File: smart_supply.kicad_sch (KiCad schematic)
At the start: 0 parts

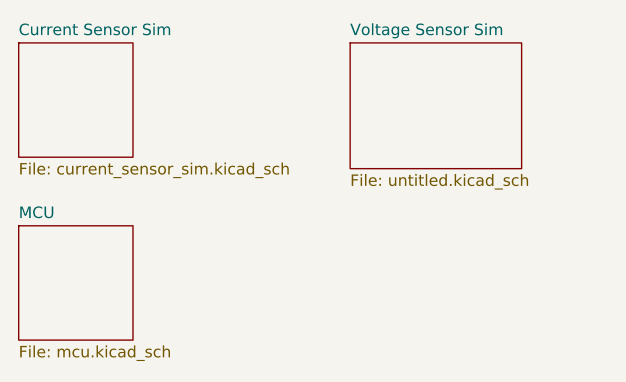
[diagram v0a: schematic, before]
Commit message: opamp chain fix
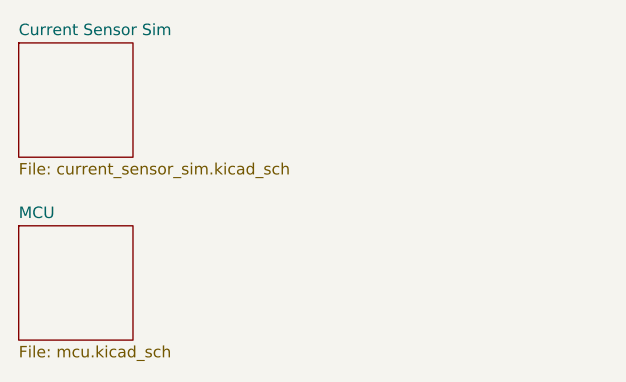
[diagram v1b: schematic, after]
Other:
- removed sheet Voltage Sensor Sim
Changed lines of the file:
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@@
-	)
-	(sheet
-		(at 59.69 21.59)
-		(size 19.05 13.97)
-		(exclude_from_sim no)
-		(in_bom yes)
-		(on_board yes)
-		(dnp no)
-		(fields_autoplaced yes)
-		(stroke
-			(width 0.1524)
-			(type solid)
-		)
-		(fill
-			(color 0 0 0 0)
-		)
-		(property "Sheetname" "Voltage Sensor Sim"
-			(at 59.69 20.8784 0)
-			(show_name no)
-			(do_not_autoplace no)
-			(effects
-				(font
-					(size 1.27 1.27)
-				)
-				(justify left bottom)
-			)
-		)
-		(property "Sheetfile" "untitled.kicad_sch"
-			(at 59.69 36.1446 0)
-			(show_name no)
-			(do_not_autoplace no)
-			(effects
-				(font
-					(size 1.27 1.27)
-				)
-				(justify left top)
-			)
-		)
-		(instances
-			(project "smart_supply"
-				(path "/487ef637-7a03-4925-80c1-798e0c6f0bbd"
-					(page "4")
-				)
-			)
-		)
 	)
 	(sheet

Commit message: built opamp network
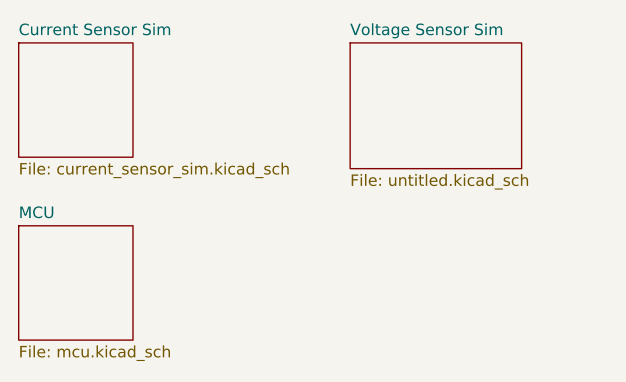
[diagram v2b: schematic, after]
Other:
- added sheet Voltage Sensor Sim (untitled.kicad_sch)
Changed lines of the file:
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@@
+	)
+	(sheet
+		(at 59.69 21.59)
+		(size 19.05 13.97)
+		(exclude_from_sim no)
+		(in_bom yes)
+		(on_board yes)
+		(dnp no)
+		(fields_autoplaced yes)
+		(stroke
+			(width 0.1524)
+			(type solid)
+		)
+		(fill
+			(color 0 0 0 0)
+		)
+		(property "Sheetname" "Voltage Sensor Sim"
+			(at 59.69 20.8784 0)
+			(show_name no)
+			(do_not_autoplace no)
+			(effects
+				(font
+					(size 1.27 1.27)
+				)
+				(justify left bottom)
+			)
+		)
+		(property "Sheetfile" "untitled.kicad_sch"
+			(at 59.69 36.1446 0)
+			(show_name no)
+			(do_not_autoplace no)
+			(effects
+				(font
+					(size 1.27 1.27)
+				)
+				(justify left top)
+			)
+		)
+		(instances
+			(project "smart_supply"
+				(path "/487ef637-7a03-4925-80c1-798e0c6f0bbd"
+					(page "4")
+				)
+			)
+		)
 	)
 	(sheet
